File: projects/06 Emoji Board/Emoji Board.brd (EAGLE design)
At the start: 59.7 x 59.7 mm, 19 parts, among them M2 MAX7219, U2 ATMEGA8A-AU-TQFP32, Y1 16MHZ

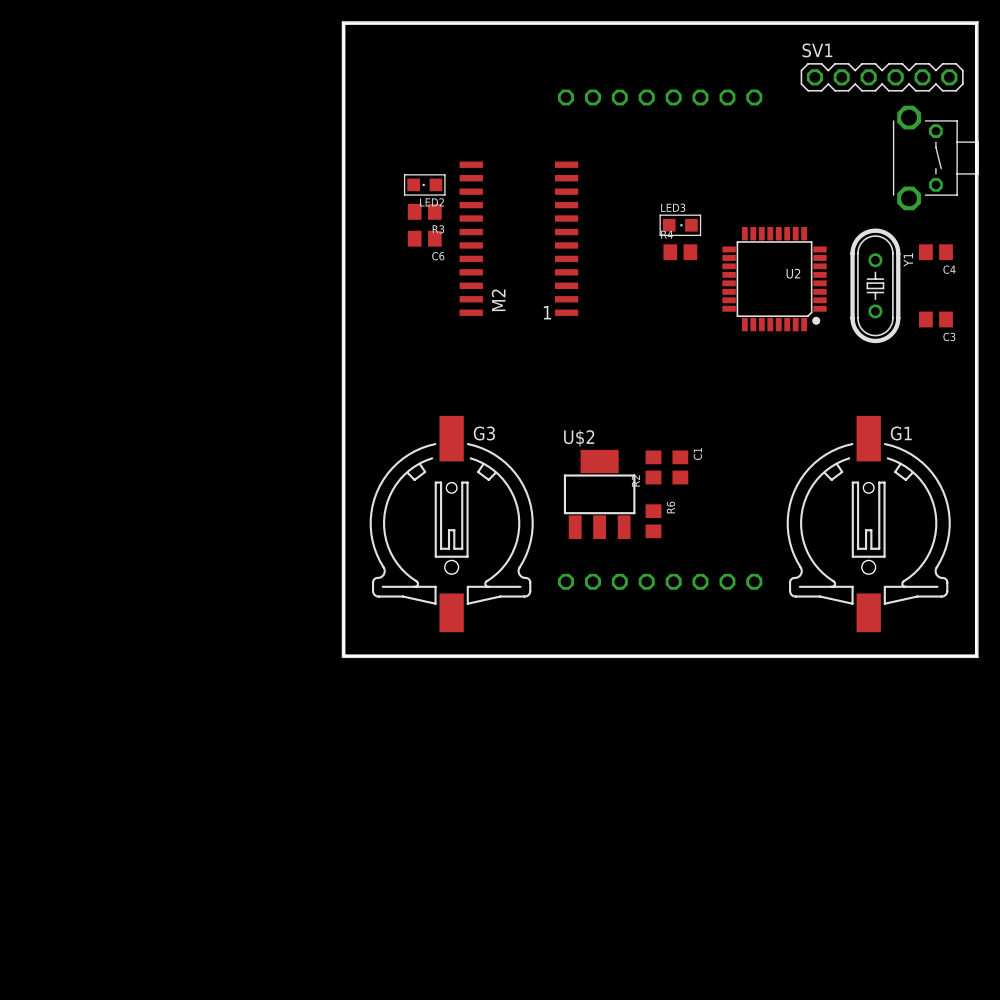
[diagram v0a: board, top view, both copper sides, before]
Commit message: 2020.06.27.01
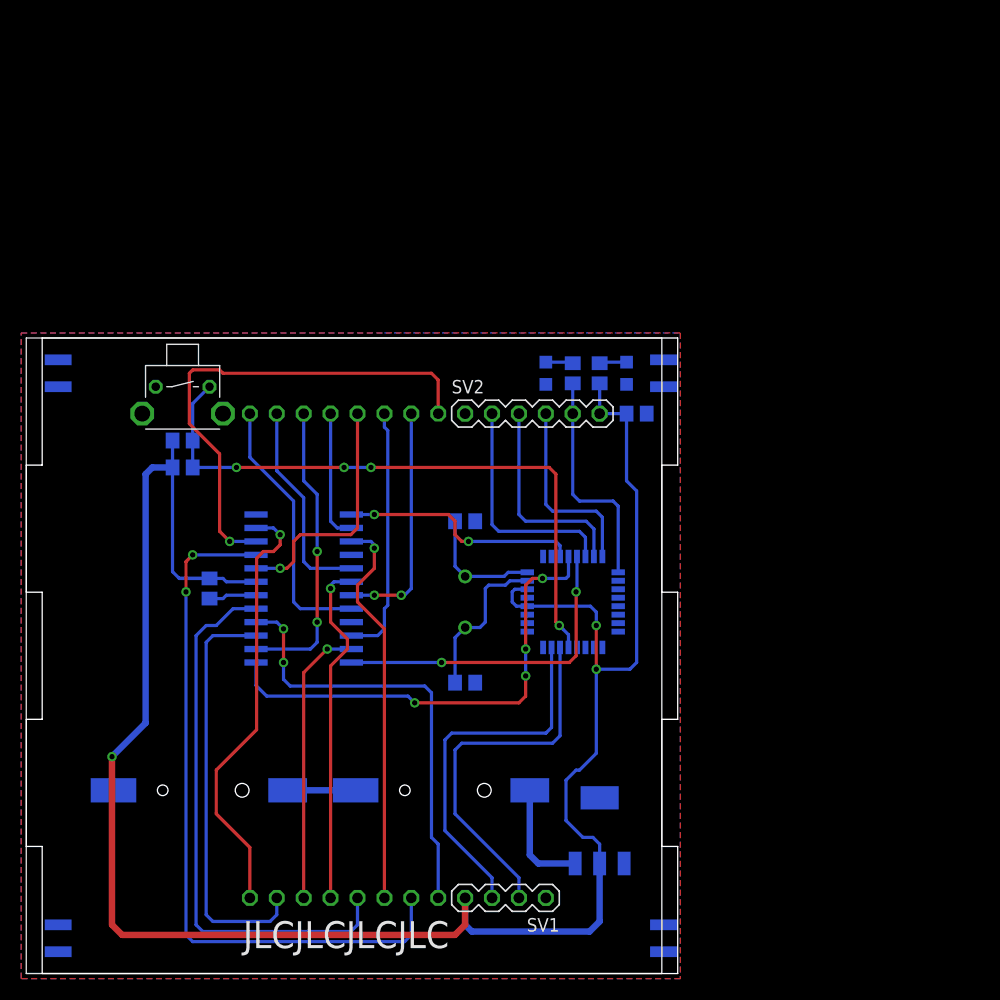
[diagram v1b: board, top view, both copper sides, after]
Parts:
- removed C6: 104, RCLDA:C0805
- removed G3: CR1220, Power:CR1220
- removed L2: DOT-MATRIX-BS2088BS, Display:2088BS
- removed LED2: GREEN, Display:CHIPLED_0805
- removed LED3: YELLOW, Display:CHIPLED_0805
- removed M2: MAX7219, Chip:SOP24
- removed R6: R0805, RCLDA:R0805
- removed U2: ATMEGA8A-AU-TQFP32, Chip:TQFP32
- removed Y1: 16MHZ, Crystal:HC49US
- added C2: C0805, RCLDA:C0805
- added G2: CR1220, Power:CR1220
- added LED1, LED4: (no value), Display:SML0805
- added R1: 103, RCLDA:R0805
- added SV2: (no value), Pin-Header:MA06-1
- added U$10, U$11, U$4, U$5, U$6, U$7, U$8, U$9: CONNECTOR, Connector:PAD
- added U$12: MAX7219, Chip:SOP24
- added U$13, U$17: (no value), Logos:5V0_050
- added U$14, U$18: (no value), Logos:GND_050
- added U$15: (no value), Logos:TXD_050
- added U$16: (no value), Logos:RXD_050
- added U$20: (no value), Logos:WWW.DIOSTUDIO.CN_100
- added U$21: (no value), Logos:LOGO_100
- added U$22: (no value), Logos:DIOSTUDIO_100
- added U$23: (no value), Logos:SCK_050
- added U$24: (no value), Logos:MISO_050
- added U$25: (no value), Logos:MOSI_050
- added U$26: (no value), Logos:SS_050
- added U$3: DOT-MATRIX-BS2088BS, Display:2088BS
- added U1: ATMEGA8A-AU-TQFP32, Chip:TQFP32
- added Y2: 16MHZ, Crystal:HC49US
- C3, C4: value 22p -> C0805
- R2: value 103 -> R0805
- R3, R4: value 471 -> R0805
- SV1: device Pin-Header:MA06-1 -> Pin-Header:MA04-1
- U$2: value (none) -> AMS1117-5V0SOT22
- moved SV1 85.2 mm to (15.2, -22.9), turned to 180 degrees
- moved U$1 74.3 mm to (-15.2, 25.4), turned to 0 degrees
- moved R4 54.6 mm to (-12.7, 6.35), flipped to the bottom, turned to 270 degrees
- moved C3 48.4 mm to (11.4, 12.7), flipped to the bottom, turned to 0 degrees
- moved C1 47.0 mm to (-15.2, 17.8), flipped to the bottom, turned to 0 degrees
- moved G1 39.2 mm to (15.2, -12.7), flipped to the bottom, turned to 270 degrees
- moved C4 32.1 mm to (27.6, 22.9), flipped to the bottom, turned to 0 degrees
- moved U$2 31.8 mm to (24.1, -16.5), flipped to the bottom
- moved R3 22.5 mm to (24.1, 26.7), flipped to the bottom, turned to 90 degrees
- moved R2 11.7 mm to (21.6, 26.7), flipped to the bottom
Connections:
- removed net D7: U2.11
- removed net D8: U2.12
- removed net D9: U2.13
- removed net N$3: C1.2, SV1.6
- net +5V: now also C1.2, C4.2, R1.1, R3.1, R4.1, SV1.4, SV2.6, U$12.19, U1.4, U1.6; no longer C6.2, M2.19, R2.1, R3.2, R6.1, SV1.3, U2.4, U2.6
- net A0: now also U1.23; no longer U2.23
- net A1: now also U1.24; no longer U2.24
- net A2: now also U1.25; no longer U2.25
- net A3: now also U1.26; no longer U2.26
- net A4: now also U1.27; no longer U2.27
- net A5: now also U1.28; no longer U2.28
- net A6: now also U1.19; no longer U2.19
- net A7: now also U1.22; no longer U2.22
- net C1: now also U$12.2, U$3.COL1; no longer L2.COL1, M2.2
- net C2: now also U$12.11, U$3.COL2; no longer L2.COL2, M2.11
- net C3: now also U$12.6, U$3.COL3; no longer L2.COL3, M2.6
- net C4: now also U$12.7, U$3.COL4; no longer L2.COL4, M2.7
- net C5: now also U$12.3, U$3.COL5; no longer L2.COL5, M2.3
- net C6: now also U$12.10, U$3.COL6; no longer L2.COL6, M2.10
- net C7: now also U$12.5, U$3.COL7; no longer L2.COL7, M2.5
- net C8: now also U$12.8, U$3.COL8; no longer L2.COL8, M2.8
- net CLK: now also U$12.13, U1.12; no longer M2.13
- net CS: now also U$12.12, U1.13; no longer M2.12
- net D2: now also U1.32; no longer U2.32
- net D3: now also U1.1; no longer U2.1
- net D4: now also U1.2; no longer U2.2
- net D5: now also U1.9; no longer U2.9
- net D6: now also U1.10; no longer U2.10
- net DIN: now also U$12.1, U1.11; no longer M2.1
- net DOUT: now also U$12.24; no longer M2.24
- net GND: now also C2.1, G2.-, LED1.C, LED4.C, SV2.1, U$12.4, U$12.9, U1.21, U1.3, U1.5; no longer C6.1, G1.-, LED2.C, LED3.C, M2.4, M2.9, SV1.2, U2.21, U2.3, U2.5
- net MISO: now also SV2.4, U1.16; no longer U2.16
- net MOSI: now also SV2.3, U1.15; no longer U2.15
- net N$1: now also LED4.A, R2.2; no longer LED3.A, R4.1
- net N$10: now also LED1.A, R3.2; no longer LED2.A, R3.1
- net N$2: now also G1.-, G2.+; no longer G1.+, G3.-
- net N$6: now also R4.2, U$12.18; no longer M2.18, R6.2
- net N$8: now also U1.20; no longer U2.20
- net N$9: now also U1.18; no longer U2.18
- net R1: now also U$12.22, U$3.ROW1; no longer L2.ROW1, M2.22
- net R2: now also U$12.14, U$3.ROW2; no longer L2.ROW2, M2.14
- net R3: now also U$12.16, U$3.ROW3; no longer L2.ROW3, M2.16
- net R4: now also U$12.20, U$3.ROW4; no longer L2.ROW4, M2.20
- net R5: now also U$12.23, U$3.ROW5; no longer L2.ROW5, M2.23
- net R6: now also U$12.21, U$3.ROW6; no longer L2.ROW6, M2.21
- net R7: now also U$12.15, U$3.ROW7; no longer L2.ROW7, M2.15
- net R8: now also U$12.17, U$3.ROW8; no longer L2.ROW8, M2.17
- net RST: now also R1.2, U1.29; no longer R2.2, U2.29
- net RXD: now also SV1.2, U1.30; no longer SV1.4, U2.30
- net SCK: now also R2.1, SV2.5, U1.17; no longer R4.2, U2.17
- net SS: now also SV2.2, U1.14; no longer U2.14
- net TXD: now also SV1.3, U1.31; no longer SV1.5, U2.31
- net VCC: now also G1.+; no longer G3.+
- net X1: now also C2.2, U1.7, Y2.2; no longer C3.2, U2.7, Y1.2
- net X2: now also C3.2, U1.8, Y2.1; no longer C4.2, U2.8, Y1.1
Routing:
- net +5V: track 0.00 -> 199.4 mm, vias 0 -> 3
- net R6: track 0.00 -> 67.4 mm, vias 0 -> 2
- net RST: track 0.00 -> 59.7 mm, vias 0 -> 4
- net R8: track 0.00 -> 52.3 mm
- net R1: track 0.00 -> 47.1 mm, vias 0 -> 1
- net CLK: track 0.00 -> 45.3 mm, vias 0 -> 4
- net R3: track 0.00 -> 41.7 mm, vias 0 -> 2
- net R5: track 0.00 -> 41.2 mm, vias 0 -> 1
- net R7: track 0.00 -> 39.5 mm
- net C5: track 0.00 -> 37.3 mm, vias 0 -> 1
- net RXD: track 0.00 -> 35.3 mm
- net TXD: track 0.00 -> 34.9 mm
- net C3: track 0.00 -> 32.9 mm, vias 0 -> 1
- net CS: track 0.00 -> 30.9 mm, vias 0 -> 2
- net R2: track 0.00 -> 28.1 mm, vias 0 -> 2
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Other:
- board size 59.7 x 59.7 mm -> 61.5 x 60 mm
- board text added: "JLCJLCJLCJLC"
